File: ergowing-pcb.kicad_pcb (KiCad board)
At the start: 2 copper layers, 150 parts, among them J1 USB_mini_micro_B, K0:0 KEYSW, K0:1 KEYSW, K0:2 KEYSW, K0:3 KEYSW, K0:4 KEYSW, K10:0 KEYSW, K10:1 KEYSW, K10:2 KEYSW, K10:3 KEYSW, K10:4 KEYSW, K11:0 KEYSW, K11:1 KEYSW, K11:2 KEYSW, K11:3 KEYSW, K11:4 KEYSW, K12:0 KEYSW, K12:1 KEYSW, K12:2 KEYSW, K12:3 KEYSW, K12:4 KEYSW, K13:0 KEYSW, K13:1 KEYSW, K13:2 KEYSW, K13:3 KEYSW, K13:4 KEYSW, K1:0 KEYSW, K1:1 KEYSW, K1:2 KEYSW, K1:3 KEYSW, K1:4 KEYSW, K2:0 KEYSW, K2:1 KEYSW, K2:2 KEYSW, K2:3 KEYSW, K2:4 KEYSW, K3:0 KEYSW, K3:1 KEYSW, K3:2 KEYSW, K3:3 KEYSW, K3:4 KEYSW, K4:0 KEYSW, K4:1 KEYSW, K4:2 KEYSW, K4:3 KEYSW, K4:4 KEYSW, K5:0 KEYSW, K5:1 KEYSW, K5:2 KEYSW, K5:3 KEYSW, K5:4 KEYSW, K6:0 KEYSW, K6:1 KEYSW, K6:3 KEYSW, K7:0 KEYSW, K7:1 KEYSW, K7:3 KEYSW, K7:4 KEYSW, K8:0 KEYSW, K8:1 KEYSW, K8:2 KEYSW, K8:3 KEYSW, K8:4 KEYSW, K9:0 KEYSW, K9:1 KEYSW, K9:2 KEYSW, K9:3 KEYSW, K9:4 KEYSW, SW1 SW_PUSH, U1 ATMEGA32U4, X1 XTAL_GND

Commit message: Layout near completion
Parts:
- K0:0, K0:1, K0:2, K0:3, K0:4: footprint keebs:Mx_Alps_150 -> keebs:Mx_Alps_150_R-5deg
- K10:0, K10:1, K10:2, K10:3, K10:4, K11:0, K11:1, K11:2, K11:3, K11:4, K12:0, K12:1, K12:2, K12:3, K12:4, K7:0, K7:4, K8:0, K8:1, K8:2, K8:3, K8:4, K9:0, K9:1, K9:2, K9:3, K9:4: footprint keebs:Mx_Alps_100 -> keebs:Mx_Alps_100_R5deg
- K13:0, K13:1, K13:2, K13:3, K13:4: footprint keebs:Mx_Alps_150 -> keebs:Mx_Alps_150_R5deg
- K1:0, K1:1, K1:2, K1:3, K1:4, K2:0, K2:1, K2:2, K2:3, K2:4, K3:0, K3:1, K3:2, K3:3, K3:4, K4:0, K4:1, K4:2, K4:3, K4:4, K5:0, K5:1, K5:2, K5:3, K6:0: footprint keebs:Mx_Alps_100 -> keebs:Mx_Alps_100_R-5deg
- moved D7:3 279.4 mm to (257.2, 347.7)
- moved D7:1 279.4 mm to (257.2, 319.1)
- moved D5:4 270.9 mm to (190.5, 376.2)
- moved D6:3 270.9 mm to (195.3, 347.7)
- moved D6:1 270.9 mm to (195.3, 319.1)
- moved D11:4 190.8 mm to (347.7, 276.2)
- moved D10:0 190.8 mm to (328.6, 200.0)
- moved D10:1 190.8 mm to (328.6, 219.1)
- moved D10:2 190.8 mm to (328.6, 238.1)
- moved D10:3 190.8 mm to (328.6, 257.2)
- moved D10:4 190.8 mm to (328.6, 276.2)
- moved D11:0 190.8 mm to (347.7, 200.0)
- moved D11:1 190.8 mm to (347.7, 216.7)
- moved D11:2 190.8 mm to (347.7, 238.1)
- moved D11:3 190.8 mm to (347.7, 257.2)
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
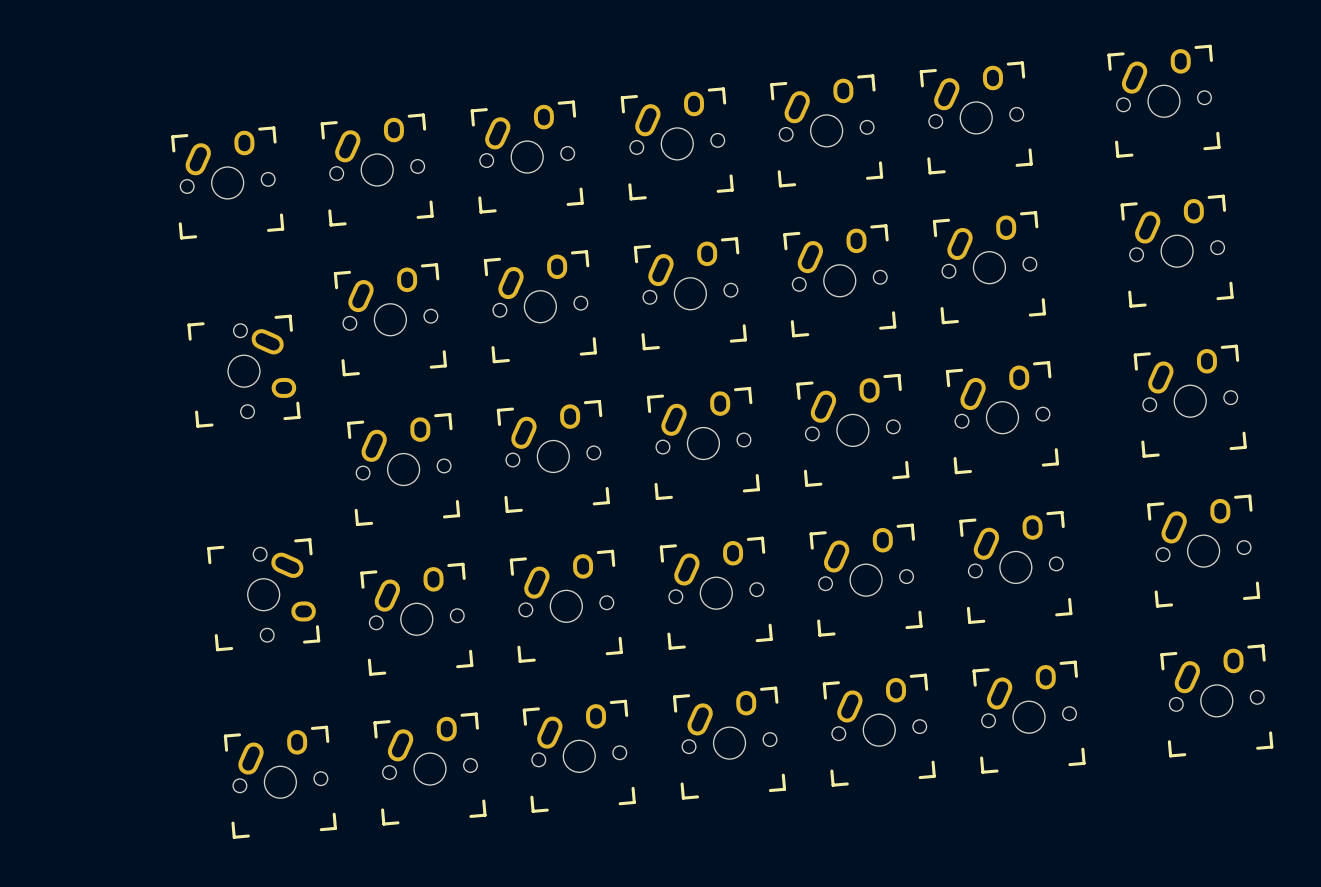
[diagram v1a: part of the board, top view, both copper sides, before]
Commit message: Layout near completion #2
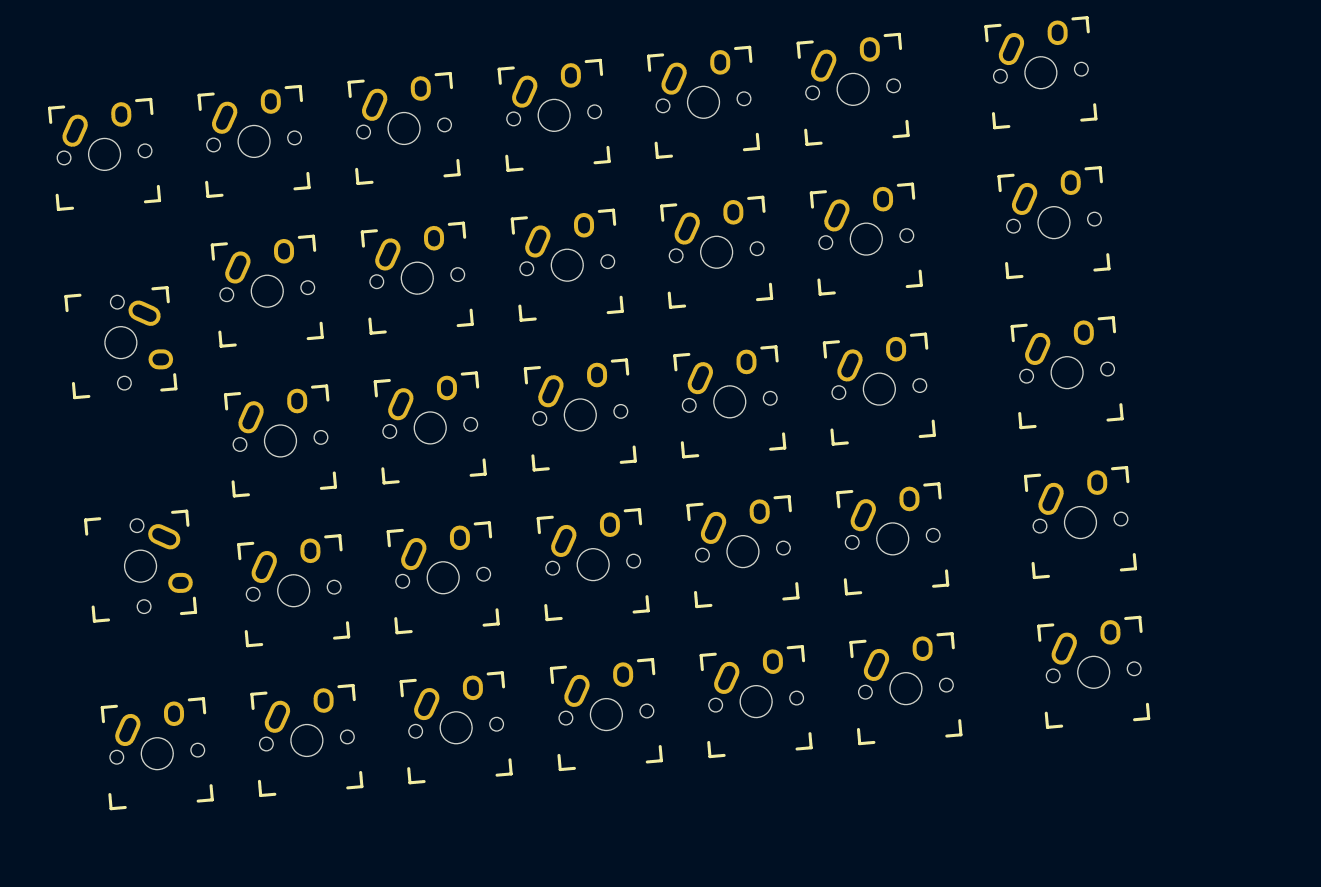
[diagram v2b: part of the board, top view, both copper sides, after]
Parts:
- moved K11:0 15.8 mm to (277.8, 43.5)
- moved K12:0 15.8 mm to (296.5, 41.8)
- moved K13:2 15.8 mm to (323.3, 77.2)
- moved K9:2 15.8 mm to (245.3, 102.9)
- moved K9:4 15.8 mm to (246.9, 121.6)
- moved K8:2 15.8 mm to (224.9, 85.8)
- moved K8:3 15.8 mm to (226.6, 104.5)
- moved K9:3 15.8 mm to (243.7, 84.2)
- moved K10:0 15.8 mm to (259.2, 45.1)
- moved K10:3 15.8 mm to (264.0, 101.2)
- moved K11:1 15.8 mm to (279.5, 62.2)
- moved K11:3 15.8 mm to (282.8, 99.6)
- moved K11:4 15.8 mm to (284.4, 118.4)
- moved K12:1 15.8 mm to (298.2, 60.5)
- moved K12:2 15.8 mm to (299.8, 79.3)
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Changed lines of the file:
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@@
     (links 515)
     (no_connects 247)
-    (area -15.201906 -10.872608 395.425 383.7146)
+    (area 43.748094 28.857392 395.425 379.0775)
     (thickness 1.6)
     (drawings 0)
@@
   )
   (module keebs:Mx_Alps_150 (layer F.Cu)
-    (at 220.39 77.06 275)
+    (at 205 73.49 275)
     (descr MXALPS)
     (tags MXALPS)
@@
   )
   (module keebs:Mx_Alps_150 (layer F.Cu)
-    (at 222.85 105 275)
+    (at 207.46 101.43 275)
     (descr MXALPS)
     (tags MXALPS)
@@
   )
   (module keebs:Mx_Alps_100_R5deg (layer F.Cu)
-    (at 218.35 53.53)
+    (at 202.96 49.96)
     (descr MXALPS)
     (tags MXALPS)
@@
   )
   (module keebs:Mx_Alps_100_R5deg (layer F.Cu)
-    (at 224.94 128.44)
+    (at 209.55 124.87)
     (descr MXALPS)
     (tags MXALPS)
@@
   )
   (module keebs:Mx_Alps_100_R5deg (layer F.Cu)
-    (at 237.04 51.91)
+    (at 221.65 48.34)
     (descr MXALPS)
     (tags MXALPS)
@@
   )
   (module keebs:Mx_Alps_100_R5deg (layer F.Cu)
-    (at 238.69 70.63)
+    (at 223.3 67.06)
     (descr MXALPS)
     (tags MXALPS)
@@
   )
   (module keebs:Mx_Alps_100_R5deg (layer F.Cu)
-    (at 240.34 89.35)
+    (at 224.95 85.78)
     (descr MXALPS)
     (tags MXALPS)
@@
   )
   (module keebs:Mx_Alps_100_R5deg (layer F.Cu)
-    (at 241.99 108.07)
+    (at 226.6 104.5)
     (descr MXALPS)
     (tags MXALPS)
@@
   )
   (module keebs:Mx_Alps_100_R5deg (layer F.Cu)
-    (at 243.64 126.79)
+    (at 228.25 123.22)
     (descr MXALPS)
     (tags MXALPS)
@@
   )
   (module keebs:Mx_Alps_100_R5deg (layer F.Cu)
-    (at 255.79 50.29)
+    (at 240.4 46.72)
     (descr MXALPS)
     (tags MXALPS)
@@
   )
   (module keebs:Mx_Alps_100_R5deg (layer F.Cu)
-    (at 257.44 69)
+    (at 242.05 65.43)
     (descr MXALPS)
     (tags MXALPS)
@@
   )
   (module keebs:Mx_Alps_100_R5deg (layer F.Cu)
-    (at 260.68 106.45)
+    (at 245.29 102.88)
     (descr MXALPS)
     (tags MXALPS)
@@
   )
   (module keebs:Mx_Alps_100_R5deg (layer F.Cu)
-    (at 259.06 87.72)
+    (at 243.67 84.15)
     (descr MXALPS)
     (tags MXALPS)
@@
   )
   (module keebs:Mx_Alps_100_R5deg (layer F.Cu)
-    (at 262.3 125.2)
+    (at 246.91 121.63)
     (descr MXALPS)
     (tags MXALPS)
@@
   )
   (module keebs:Mx_Alps_100_R5deg (layer F.Cu)
-    (at 274.55 48.65)
+    (at 259.16 45.08)
     (descr MXALPS)
     (tags MXALPS)
@@
   )
   (module keebs:Mx_Alps_100_R5deg (layer F.Cu)
-    (at 276.19 67.38)
+    (at 260.8 63.81)
     (descr MXALPS)
     (tags MXALPS)
@@
   )
   (module keebs:Mx_Alps_100_R5deg (layer F.Cu)
-    (at 277.82 86.1)
+    (at 262.43 82.53)
     (descr MXALPS)
     (tags MXALPS)
@@
   )
   (module keebs:Mx_Alps_100_R5deg (layer F.Cu)
-    (at 279.43 104.81)
+    (at 264.04 101.24)
     (descr MXALPS)
     (tags MXALPS)
@@
   )
   (module keebs:Mx_Alps_100_R5deg (layer F.Cu)
-    (at 281.08 123.55)
+    (at 265.69 119.98)
     (descr MXALPS)
     (tags MXALPS)
@@
   )
   (module keebs:Mx_Alps_100_R5deg (layer F.Cu)
-    (at 293.22 47.02)
+    (at 277.83 43.45)
     (descr MXALPS)
     (tags MXALPS)
@@
   )
   (module keebs:Mx_Alps_100_R5deg (layer F.Cu)
-    (at 294.86 65.76)
+    (at 279.47 62.19)
     (descr MXALPS)
     (tags MXALPS)
@@
   )
   (module keebs:Mx_Alps_100_R5deg (layer F.Cu)
-    (at 296.5 84.46)
+    (at 281.11 80.89)
     (descr MXALPS)
     (tags MXALPS)
@@
   )
   (module keebs:Mx_Alps_100_R5deg (layer F.Cu)
-    (at 298.15 103.18)
+    (at 282.76 99.61)
     (descr MXALPS)
     (tags MXALPS)
@@
   )
   (module keebs:Mx_Alps_100_R5deg (layer F.Cu)
-    (at 299.8 121.93)
+    (at 284.41 118.36)
     (descr MXALPS)
     (tags MXALPS)
@@
   )
   (module keebs:Mx_Alps_100_R5deg (layer F.Cu)
-    (at 311.92 45.4)
+    (at 296.53 41.83)
     (descr MXALPS)
     (tags MXALPS)
@@
   )
   (module keebs:Mx_Alps_100_R5deg (layer F.Cu)
-    (at 313.57 64.12)
+    (at 298.18 60.55)
     (descr MXALPS)
     (tags MXALPS)
@@
   )
   (module keebs:Mx_Alps_100_R5deg (layer F.Cu)
-    (at 315.2 82.87)
+    (at 299.81 79.3)
     (descr MXALPS)
     (tags MXALPS)
@@
   )
   (module keebs:Mx_Alps_100_R5deg (layer F.Cu)
-    (at 318.52 120.31)
+    (at 303.13 116.74)
     (descr MXALPS)
     (tags MXALPS)
@@
   )
   (module keebs:Mx_Alps_100_R5deg (layer F.Cu)
-    (at 316.87 101.59)
+    (at 301.48 98.02)
     (descr MXALPS)
     (tags MXALPS)
@@
   )
   (module keebs:Mx_Alps_150_R5deg (layer F.Cu)
-    (at 335.39 43.32)
+    (at 320 39.75)
     (descr MXALPS)
     (tags MXALPS)
@@
   )
   (module keebs:Mx_Alps_150_R5deg (layer F.Cu)
-    (at 337.03 62.06)
+    (at 321.64 58.49)
     (descr MXALPS)
     (tags MXALPS)
@@
   )
   (module keebs:Mx_Alps_150_R5deg (layer F.Cu)
-    (at 338.67 80.81)
+    (at 323.28 77.24)
     (descr MXALPS)
     (tags MXALPS)
@@
   )
   (module keebs:Mx_Alps_150_R5deg (layer F.Cu)
-    (at 340.34 99.55)
+    (at 324.95 95.98)
     (descr MXALPS)
     (tags MXALPS)
@@
   )
   (module keebs:Mx_Alps_150_R5deg (layer F.Cu)
-    (at 341.99 118.27)
+    (at 326.6 114.7)
     (descr MXALPS)
     (tags MXALPS)
